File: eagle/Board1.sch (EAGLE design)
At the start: 3 parts

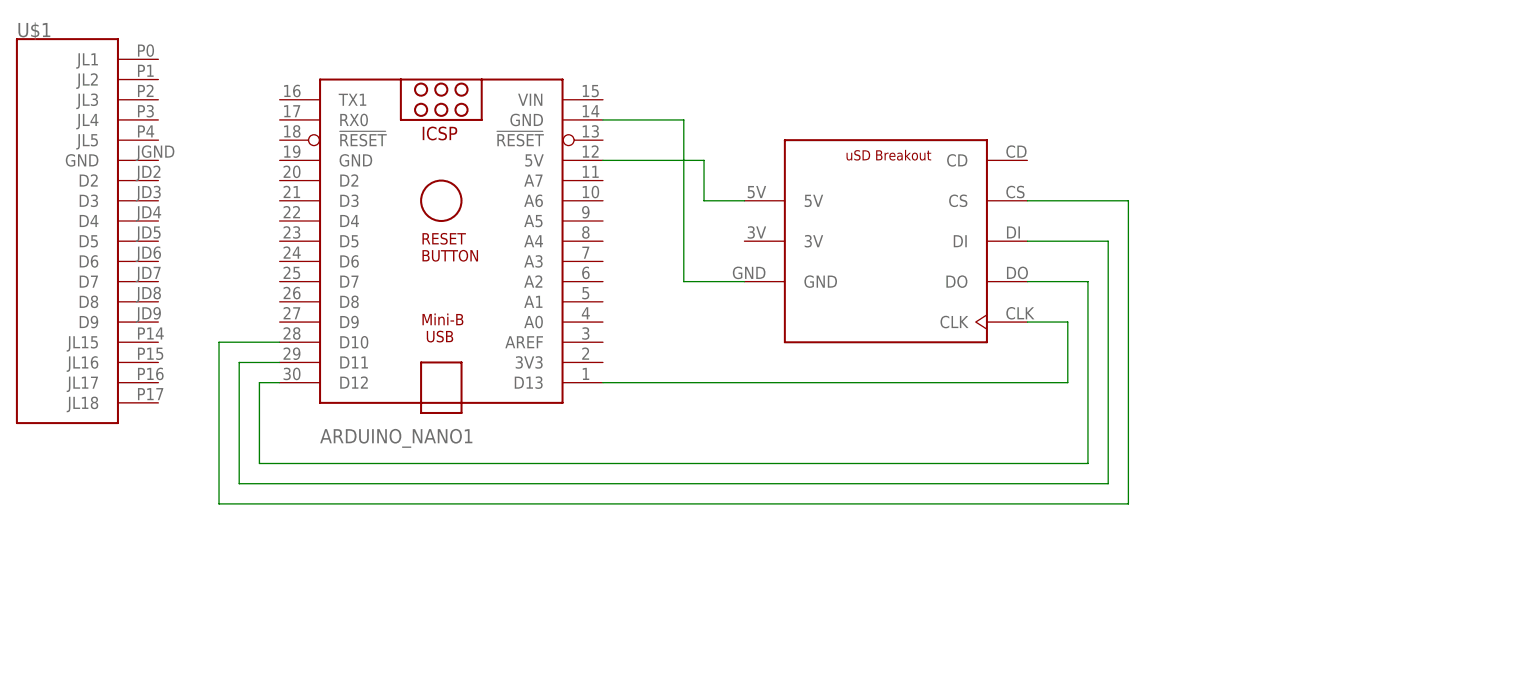
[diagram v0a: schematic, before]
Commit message: Board 1 nearly complete
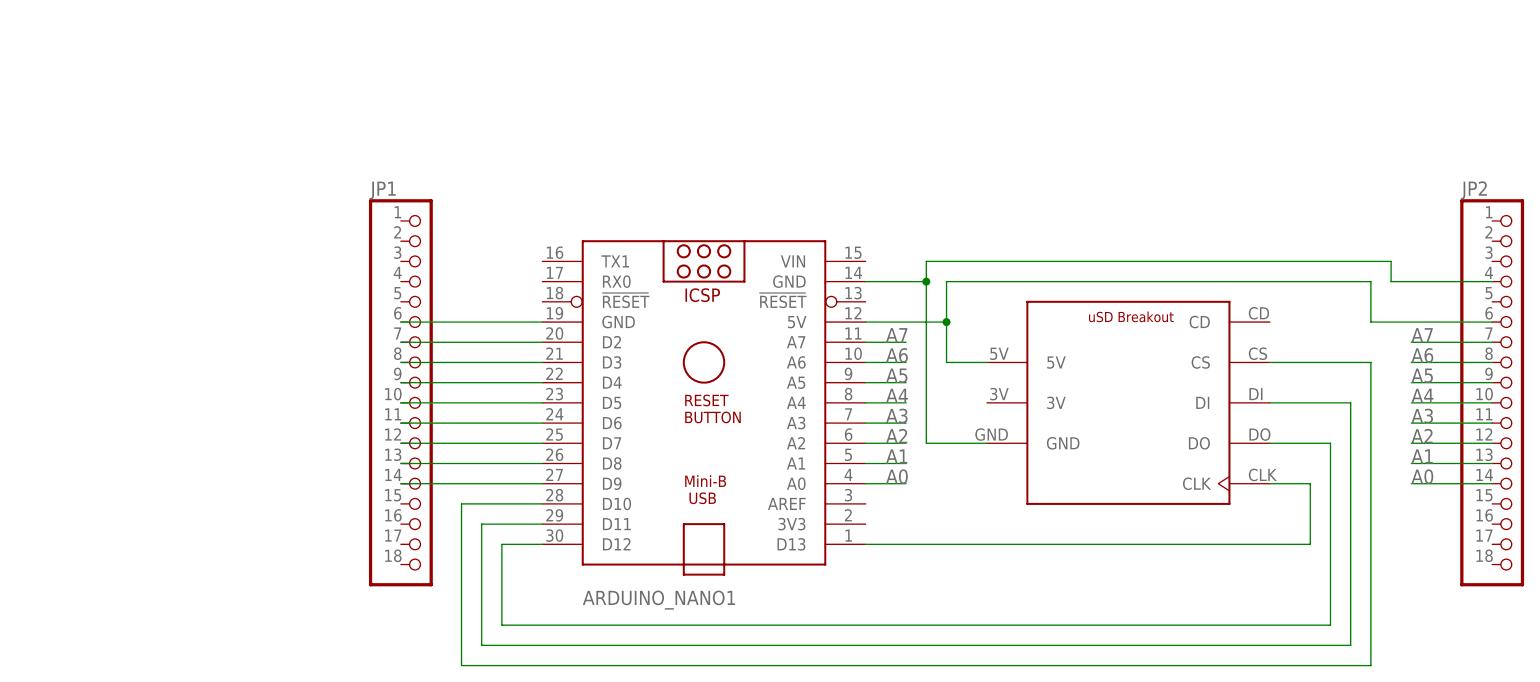
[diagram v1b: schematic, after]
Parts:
- removed U$1: JLEFT, cwParts:JLEFT
- added JP1, JP2: (no value), pinhead:PINHD-1X18
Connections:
- new net A0: ARDUINO_NANO1.A0, JP2.14
- new net A1: ARDUINO_NANO1.A1, JP2.13
- new net A2: ARDUINO_NANO1.A2, JP2.12
- new net A3: ARDUINO_NANO1.A3, JP2.11
- new net A4: ARDUINO_NANO1.A4, JP2.10
- new net A5: ARDUINO_NANO1.A5, JP2.9
- new net A6: ARDUINO_NANO1.A6, JP2.8
- new net A7: ARDUINO_NANO1.A7, JP2.7
- new net N$10: ARDUINO_NANO1.D6, JP1.11
- new net N$11: ARDUINO_NANO1.D5, JP1.10
- new net N$12: ARDUINO_NANO1.D4, JP1.9
- new net N$13: ARDUINO_NANO1.D3, JP1.8
- new net N$14: ARDUINO_NANO1.D2, JP1.7
- new net N$15: ARDUINO_NANO1.GND@1, JP1.6
- new net N$7: ARDUINO_NANO1.D9, JP1.14
- new net N$8: ARDUINO_NANO1.D8, JP1.13
- new net N$9: ARDUINO_NANO1.D7, JP1.12
- net N$1: now also JP2.4
- net N$2: now also JP2.6
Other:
- moved on the sheet: ARDUINO_NANO1
